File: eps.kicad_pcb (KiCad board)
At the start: 2 copper layers, 90 x 96 mm, 52 parts, among them J1 Barrel_Jack, J2 Conn_01x02_Pin, J3 Conn_01x02_Pin, J4 Conn_01x02_Pin, J5 Conn_01x02_Pin, J6 Conn_01x02_Pin, U1 LT3652EMSE, U2 INA234AxYBJ, U3 INA234AxYBJ

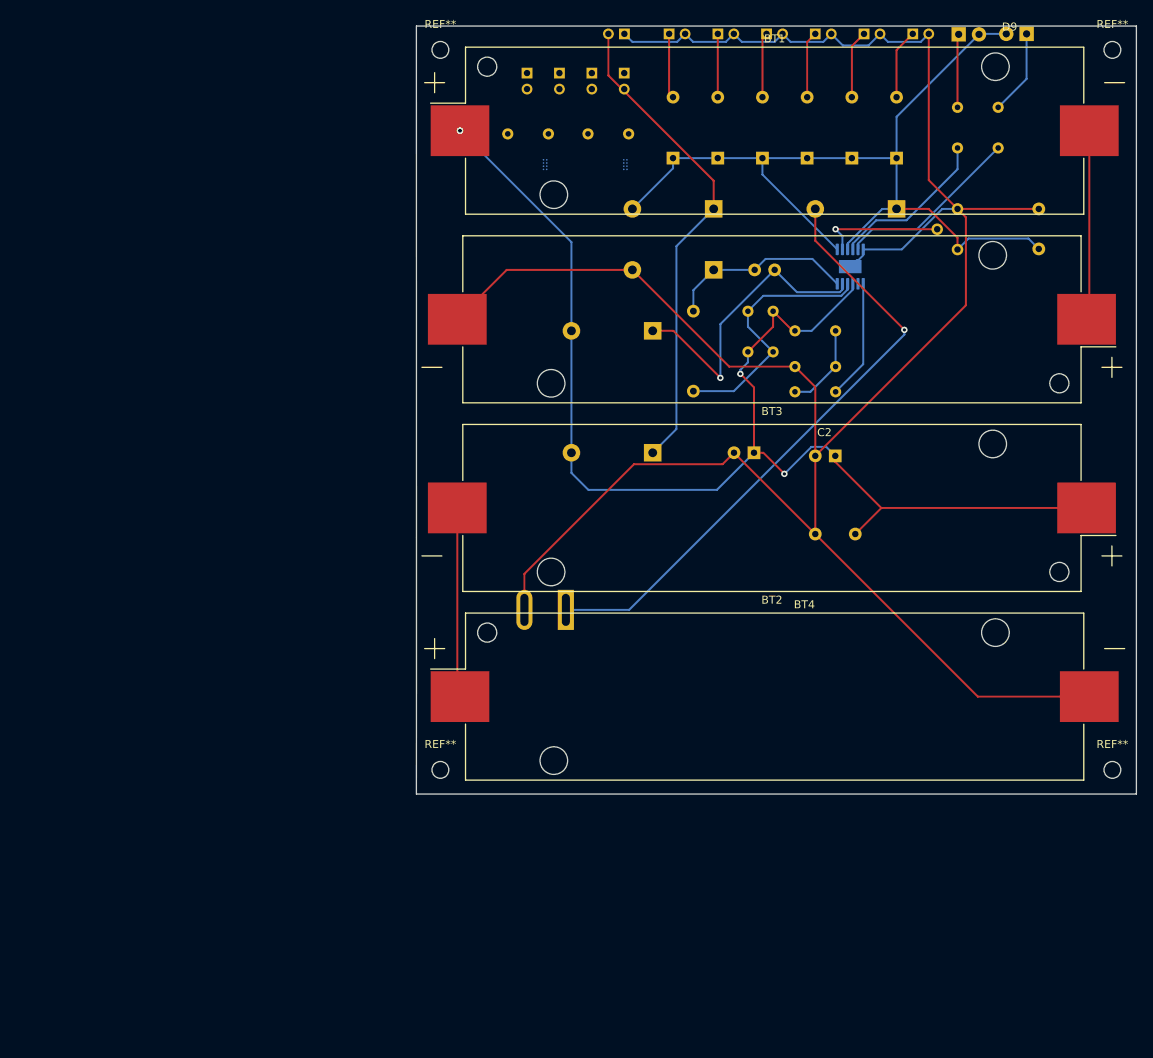
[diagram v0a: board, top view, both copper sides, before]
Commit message: new design
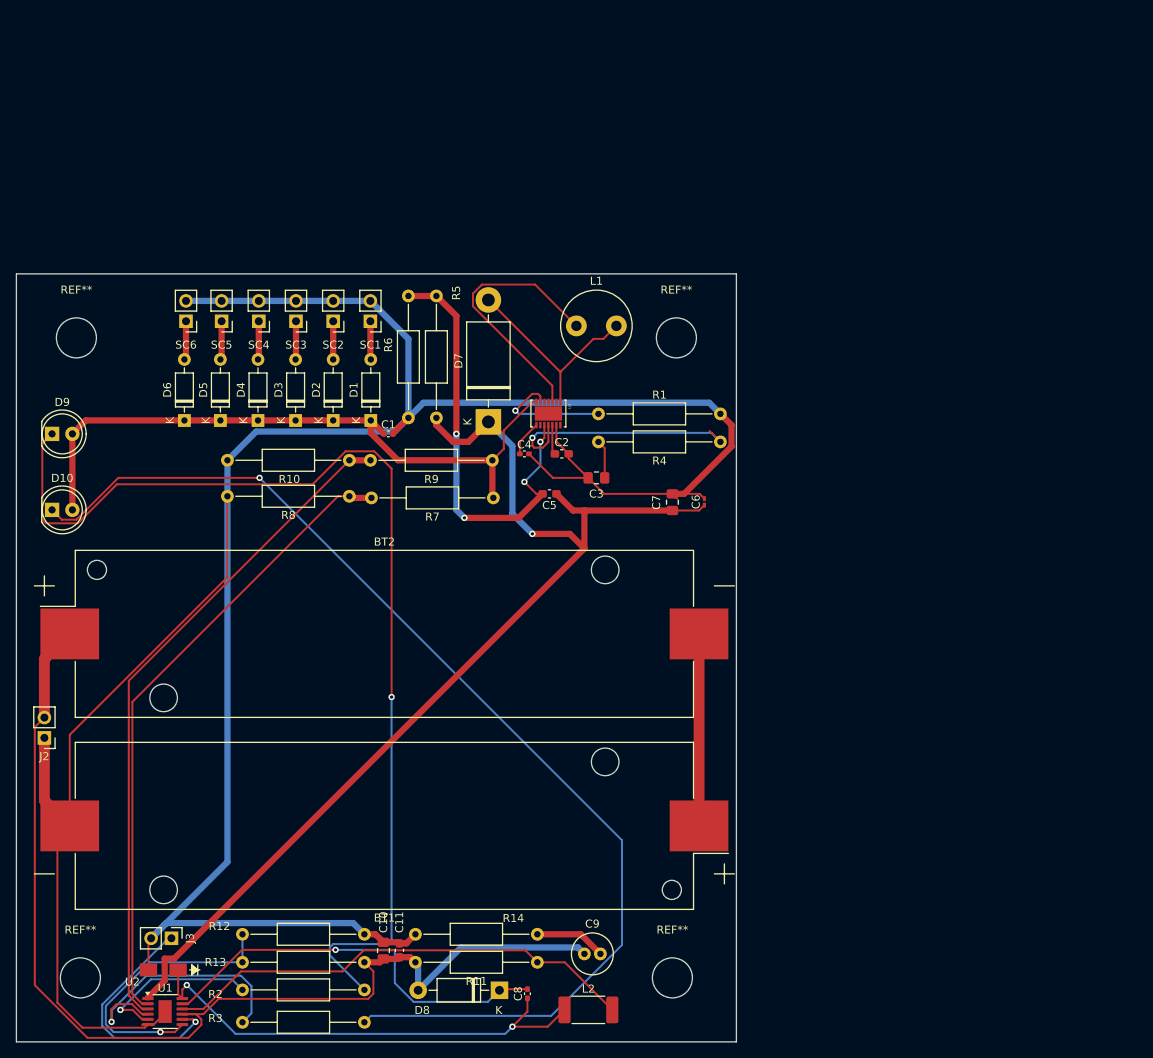
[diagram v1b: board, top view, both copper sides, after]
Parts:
- removed BT3, BT4: Battery_Cell, Battery:BatteryHolder_Keystone_1042_1x18650
- removed D11, D12, D13: 1N5819, Diode_THT:D_DO-41_SOD81_P10.16mm_Horizontal
- removed J1: Barrel_Jack, Connector_BarrelJack:BarrelJack_SwitchcraftConxall_RAPC10U_Horizontal
- removed J4, J5, J6: Conn_01x02_Pin, Connector_PinHeader_2.00mm:PinHeader_1x02_P2.00mm_Vertical
- removed the REF** at (103.0, 126.0)
- removed the REF** at (187.0, 126.0)
- removed the REF** at (187.0, 36.0)
- removed the REF** at (103.0, 36.0)
- removed RV1: 10k, Potentiometer_THT:Potentiometer_Bourns_3386P_Vertical
- added C10: 10uF 16V, Capacitor_SMD:C_0805_2012Metric_Pad1.18x1.45mm_HandSolder, F.Cu at (95.9, 148.6)
- added C11: 1uF, Capacitor_SMD:C_0603_1608Metric_Pad1.08x0.95mm_HandSolder, F.Cu at (97.9, 148.6)
- added C6: 0.1uF 10V, Capacitor_SMD:C_0201_0603Metric_Pad0.64x0.40mm_HandSolder, F.Cu at (136.0, 92.5)
- added C7: 10uF 10V, Capacitor_SMD:C_0805_2012Metric_Pad1.18x1.45mm_HandSolder, F.Cu at (132.0, 92.5)
- added C8: 1uF 50V, Capacitor_SMD:C_0402_1005Metric_Pad0.74x0.62mm_HandSolder, F.Cu at (113.9, 154.0)
- added C9: 100uF 10V, Capacitor_THT:C_Radial_D5.0mm_H11.0mm_P2.00mm, F.Cu at (121.0, 149.0)
- added L2: 10uH, Inductor_SMD:L_2512_6332Metric_Pad1.52x3.35mm_HandSolder, F.Cu at (121.5, 156.0)
- added R10: 100k, Resistor_THT:R_Axial_DIN0207_L6.3mm_D2.5mm_P15.24mm_Horizontal, F.Cu at (91.6, 87.3)
- added R11: 0.068, Resistor_THT:R_Axial_DIN0207_L6.3mm_D2.5mm_P15.24mm_Horizontal, F.Cu at (115.1, 150.1)
- added R12: 430k, Resistor_THT:R_Axial_DIN0207_L6.3mm_D2.5mm_P15.24mm_Horizontal, F.Cu at (78.3, 146.6)
- added R13: 606k, Resistor_THT:R_Axial_DIN0207_L6.3mm_D2.5mm_P15.24mm_Horizontal, F.Cu at (78.3, 150.1)
- added R14: 0.1, Resistor_THT:R_Axial_DIN0207_L6.3mm_D2.5mm_P15.24mm_Horizontal, F.Cu at (115.1, 146.6)
- added REF**: MountingHole_5mm, MountingHole:MountingHole_5mm, F.Cu at (132.0, 152.0)
- added REF**: MountingHole_5mm, MountingHole:MountingHole_5mm, F.Cu at (58.0, 152.0)
- added REF**: MountingHole_5mm, MountingHole:MountingHole_5mm, F.Cu at (132.5, 72.0)
- added REF**: MountingHole_5mm, MountingHole:MountingHole_5mm, F.Cu at (57.5, 72.0)
- BT1, BT2: value Battery_Cell -> 3.7v
- C1: value 10uF -> 2.2uF; footprint Capacitor_THT:C_Disc_D5.1mm_W3.2mm_P5.00mm -> Capacitor_SMD:C_0402_1005Metric_Pad0.74x0.62mm_HandSolder; moved to F.Cu
- C2: value 100uF -> 0.1uF; footprint Capacitor_THT:CP_Radial_D6.3mm_P2.50mm -> Capacitor_SMD:C_0603_1608Metric_Pad1.08x0.95mm_HandSolder; moved to F.Cu
- C3: value 1uF -> 10nF; footprint Capacitor_THT:C_Disc_D5.0mm_W2.5mm_P2.50mm -> Capacitor_SMD:C_0805_2012Metric_Pad1.18x1.45mm_HandSolder; moved to F.Cu
- C4: value 10uF -> 100pF; footprint Capacitor_THT:C_Disc_D5.1mm_W3.2mm_P5.00mm -> Capacitor_SMD:C_0402_1005Metric_Pad0.74x0.62mm_HandSolder; moved to F.Cu
- C5: value 100uF 16v -> 470pF; footprint Capacitor_THT:CP_Radial_D6.3mm_P2.50mm -> Capacitor_SMD:C_0603_1608Metric_Pad1.08x0.95mm_HandSolder; moved to F.Cu
- D1, D2, D3, D4, D5, D6: moved to F.Cu
- D10, D9: footprint LED_THT:LED_Rectangular_W3.0mm_H2.0mm -> LED_THT:LED_D5.0mm; moved to F.Cu
- D7: value 1N5819 -> MBR340; footprint Diode_THT:D_DO-41_SOD81_P10.16mm_Horizontal -> Diode_THT:D_DO-201AD_P15.24mm_Horizontal; moved to F.Cu
- D8: value 1N5819 -> 1N5817; moved to F.Cu
- J2: value Conn_01x02_Pin -> Out-; footprint Connector_PinHeader_2.00mm:PinHeader_1x02_P2.00mm_Vertical -> Connector_PinHeader_2.54mm:PinHeader_1x02_P2.54mm_Vertical; moved to F.Cu
- J3: value Conn_01x02_Pin -> NTC_PIN; footprint Connector_PinHeader_2.00mm:PinHeader_1x02_P2.00mm_Vertical -> Connector_PinHeader_2.54mm:PinHeader_1x02_P2.54mm_Vertical; moved to F.Cu
- L1: value 68uH -> 4.7uH; footprint Inductor_THT:L_Axial_L5.0mm_D3.6mm_P10.00mm_Horizontal_Murata_BL01RN1A2A2 -> Inductor_THT:L_Radial_D8.7mm_P5.00mm_Fastron_07HCP; moved to F.Cu
- R1: value 568k -> 17.8k; footprint Resistor_THT:R_Axial_DIN0204_L3.6mm_D1.6mm_P5.08mm_Horizontal -> Resistor_THT:R_Axial_DIN0207_L6.3mm_D2.5mm_P15.24mm_Horizontal; moved to F.Cu
- R2, R3: footprint Resistor_THT:R_Axial_DIN0204_L3.6mm_D1.6mm_P5.08mm_Horizontal -> Resistor_THT:R_Axial_DIN0207_L6.3mm_D2.5mm_P15.24mm_Horizontal; moved to F.Cu
- R4: value 0.22 -> 4.32k; footprint Resistor_THT:R_Axial_DIN0204_L3.6mm_D1.6mm_P5.08mm_Horizontal -> Resistor_THT:R_Axial_DIN0207_L6.3mm_D2.5mm_P15.24mm_Horizontal; moved to F.Cu
- R5: value 0.5 -> 200k; footprint Resistor_THT:R_Axial_DIN0204_L3.6mm_D1.6mm_P5.08mm_Horizontal -> Resistor_THT:R_Axial_DIN0207_L6.3mm_D2.5mm_P15.24mm_Horizontal; moved to F.Cu
- R6: value 446k -> 23.2k; footprint Resistor_THT:R_Axial_DIN0204_L3.6mm_D1.6mm_P5.08mm_Horizontal -> Resistor_THT:R_Axial_DIN0207_L6.3mm_D2.5mm_P15.24mm_Horizontal; moved to F.Cu
- R7: value 200k -> 38.3k; footprint Resistor_THT:R_Axial_DIN0204_L3.6mm_D1.6mm_P5.08mm_Horizontal -> Resistor_THT:R_Axial_DIN0207_L6.3mm_D2.5mm_P15.24mm_Horizontal; moved to F.Cu
- R8: value R -> 100k; footprint Resistor_THT:R_Axial_DIN0204_L3.6mm_D1.6mm_P5.08mm_Horizontal -> Resistor_THT:R_Axial_DIN0207_L6.3mm_D2.5mm_P15.24mm_Horizontal; moved to F.Cu
- R9: value R -> 210k; footprint Resistor_THT:R_Axial_DIN0204_L3.6mm_D1.6mm_P5.08mm_Horizontal -> Resistor_THT:R_Axial_DIN0207_L6.3mm_D2.5mm_P15.24mm_Horizontal; moved to F.Cu
- SC1, SC2, SC3, SC4, SC5, SC6: footprint Connector_PinHeader_2.00mm:PinHeader_1x02_P2.00mm_Vertical -> Connector_PinHeader_2.54mm:PinHeader_1x02_P2.54mm_Vertical; moved to F.Cu
- U1: value LT3652EMSE -> LT3652IMSE; moved to F.Cu
- U2: value INA234AxYBJ -> CMSH3-40MA; footprint Package_BGA:Texas_DSBGA-8_0.705x1.468mm_Layout2x4_P0.4mm -> CMSH3-40MA:SMA; moved to F.Cu
- U3: value INA234AxYBJ -> LT3479EDE_TRPBF; footprint Package_BGA:Texas_DSBGA-8_0.705x1.468mm_Layout2x4_P0.4mm -> LT3479EDE_TRPBF:DFN-14_DE; moved to F.Cu
- moved R2 141.4 mm to (78.3, 153.5), turned to 0 degrees
- moved R3 141.2 mm to (78.3, 157.6), turned to 0 degrees
- moved D9 131.7 mm to (54.5, 84.0), turned to 0 degrees
- moved D10 128.0 mm to (54.5, 93.5)
- moved U1 126.5 mm to (68.6, 156.2), turned to 0 degrees
- moved J3 122.1 mm to (69.4, 147.1), turned to -90 degrees
- moved U2 116.1 mm to (68.4, 151.0)
- moved J2 114.0 mm to (53.5, 122.0), turned to 180 degrees
- moved BT1 99.7 mm to (96.0, 133.0), turned to 180 degrees
- moved SC6 97.7 mm to (71.2, 69.9), turned to 180 degrees
- moved D6 94.9 mm to (71.0, 82.3)
- moved D8 93.9 mm to (110.4, 153.6)
- moved SC5 88.0 mm to (75.7, 69.9), turned to 180 degrees
- moved D5 85.5 mm to (75.5, 82.3)
- moved C1 84.5 mm to (96.5, 84.0), turned to 0 degrees
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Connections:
- BT1 pad 2: Net-(BT1--) -> GND
- BT2 pad 1: Net-(BT1-+) -> +5V
- BT2 pad 2: Net-(BT2--) -> Net-(BT1-+)
- C2 pad 1: Net-(BT1-+) -> Net-(U3-SS)
- C3 pad 1: Net-(D11-K) -> Net-(C3-Pad1)
- C3 pad 2: Net-(D8-K) -> GND
- C4 pad 1: Net-(BT1-+) -> Net-(U3-FBP)
- C5 pad 1: Net-(BT1-+) -> Net-(D7-K)
- C5 pad 2: GND -> Net-(U3-FBN)
- D1 pad 1: /Power sensor/source -> /BatteryCharger/in
- D2 pad 1: /Power sensor/source -> /BatteryCharger/in
- D3 pad 1: /Power sensor/source -> /BatteryCharger/in
- D4 pad 1: /Power sensor/source -> /BatteryCharger/in
- D5 pad 1: /Power sensor/source -> /BatteryCharger/in
- D6 pad 1: /Power sensor/source -> /BatteryCharger/in
- D7 pad 1: /BatteryCharger/in -> Net-(D7-K)
- D8 pad 2: GND -> +5V
- J3 pad 1: /Power sensor/scl -> Net-(J3-Pin_1)
- J3 pad 2: /Power sensor/sda -> GND
- L1 pad 1: Net-(D8-K) -> Net-(U3-L)
- L1 pad 2: Net-(U1-SENSE) -> Net-(D7-A)
- R1 pad 1: Net-(BT1-+) -> Net-(U3-RT)
- R1 pad 2: Net-(R1-Pad2) -> GND
- R4 pad 1: Net-(U1-SENSE) -> Net-(U3-VC)
- R4 pad 2: Net-(BT1-+) -> Net-(C3-Pad1)
- R5 pad 1: Net-(BT1-+) -> Net-(D7-K)
- R5 pad 2: Net-(U1-SENSE) -> Net-(U3-FBN)
- R6 pad 1: Net-(R1-Pad2) -> Net-(U3-FBN)
- R7 pad 1: Net-(U1-V_{FB}) -> /BatteryCharger/in
- R7 pad 2: Net-(R1-Pad2) -> Net-(U1-V_{IN_REG})
- R8 pad 1: Net-(D13-A) -> Net-(U1-V_{IN_REG})
- R8 pad 2: Net-(BT1-+) -> GND
- R9 pad 1: /Power sensor/source -> /BatteryCharger/in
- R9 pad 2: /BatteryCharger/in -> Net-(U1-~{SHDN})
- U1 pad 1: /BatteryCharger/in -> Net-(D7-K)
- U1 pad 11: Net-(D11-K) -> Net-(D8-K)
- U1 pad 12: Net-(D8-K) -> Net-(U1-SW)
- U1 pad 3: /BatteryCharger/in -> Net-(U1-~{SHDN})
- U1 pad 8: unconnected-(U1-NTC-Pad8) -> Net-(J3-Pin_1)
- U1 pad 9: Net-(BT1-+) -> +5V
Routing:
- net Net-(BT1-+): track 163.0 -> 24.0 mm, vias 4 -> 0
- net Net-(D7-K): track 0.00 -> 136.6 mm, vias 0 -> 1
- net Net-(D10-K): track 9.18 -> 142.0 mm, vias 0 -> 1
- net Net-(D9-K): track 10.7 -> 133.8 mm, vias 0 -> 1
- net Net-(U1-~{SHDN}): track 0.00 -> 84.1 mm
- net +5V: track 61.0 -> 136.5 mm
- net Net-(U1-V_{IN_REG}): track 15.6 -> 79.6 mm, vias 1 -> 0
- net Net-(U1-SW): track 0.00 -> 61.0 mm, vias 0 -> 2
- net GND: track 300.9 -> 359.4 mm
- net Net-(U3-FBN): track 0.00 -> 54.7 mm, vias 0 -> 4
- net Net-(D7-A): track 76.9 -> 25.9 mm, vias 1 -> 0
- net Net-(D11-K): track 37.7 -> 0.00 mm, vias 1 -> 0
- net Net-(U3-L): track 0.00 -> 33.2 mm
- net Net-(U3-VC): track 0.00 -> 31.7 mm, vias 0 -> 1
- net Net-(J3-Pin_1): track 0.00 -> 29.7 mm, vias 0 -> 1
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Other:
- outline, holes or cut-outs redrawn
- board text removed: "Hydrogen v0.1"
- board text removed: "Ulog3"
